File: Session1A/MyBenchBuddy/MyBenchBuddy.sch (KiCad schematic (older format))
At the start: 0 parts

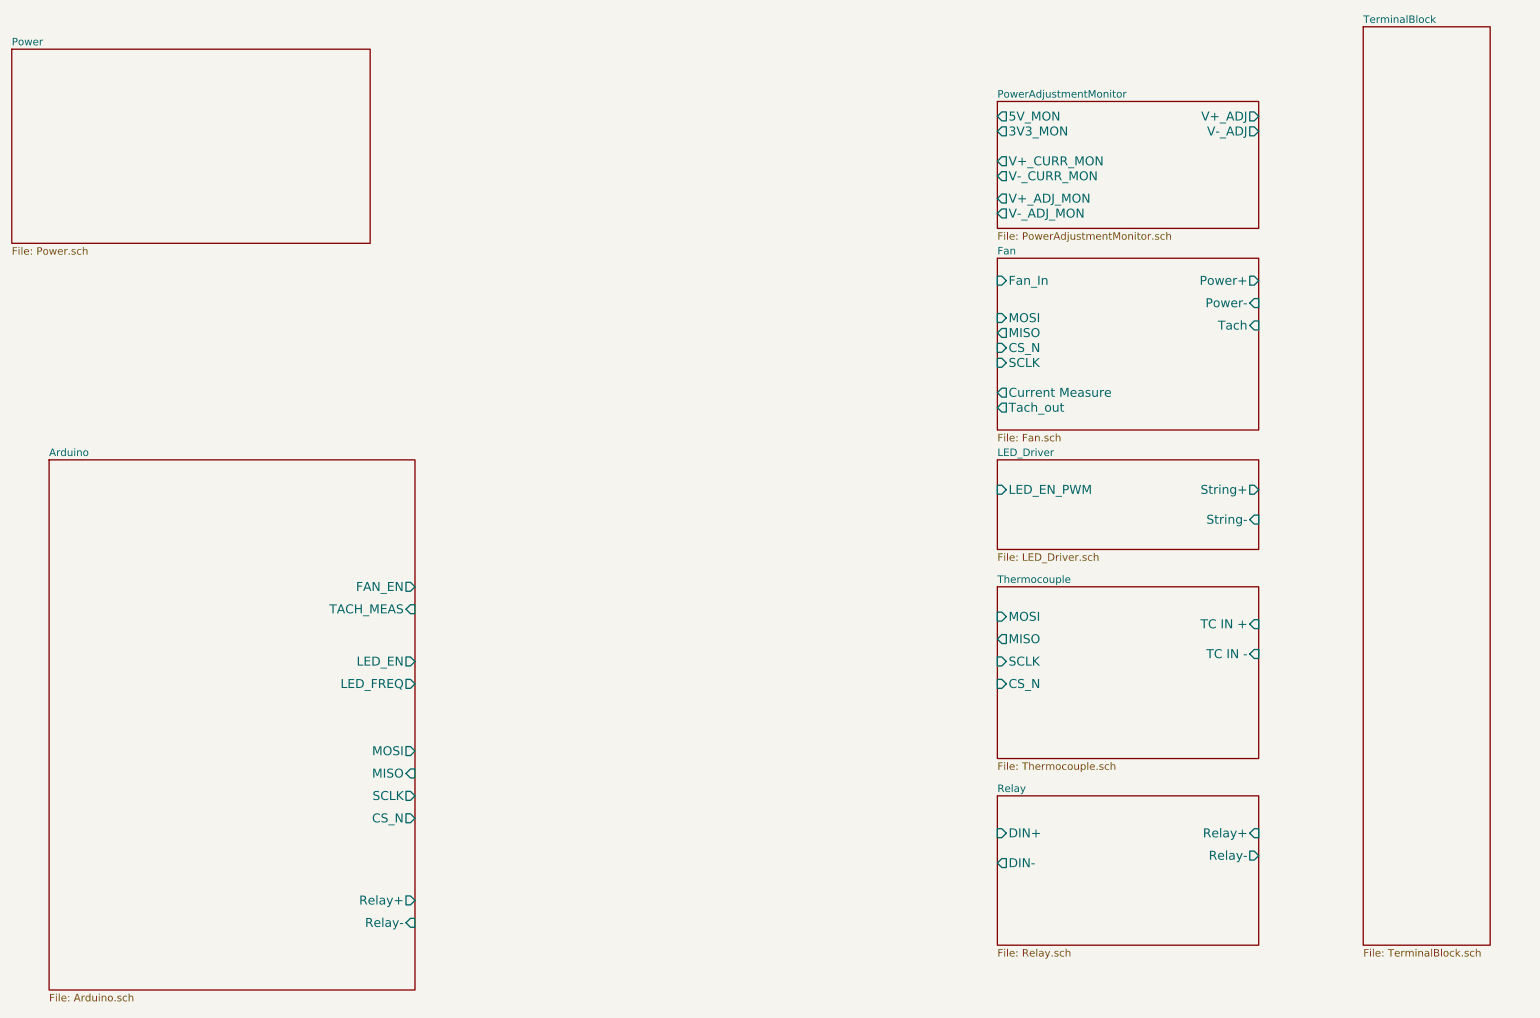
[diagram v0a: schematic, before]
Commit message: Understanding the Arduino Module
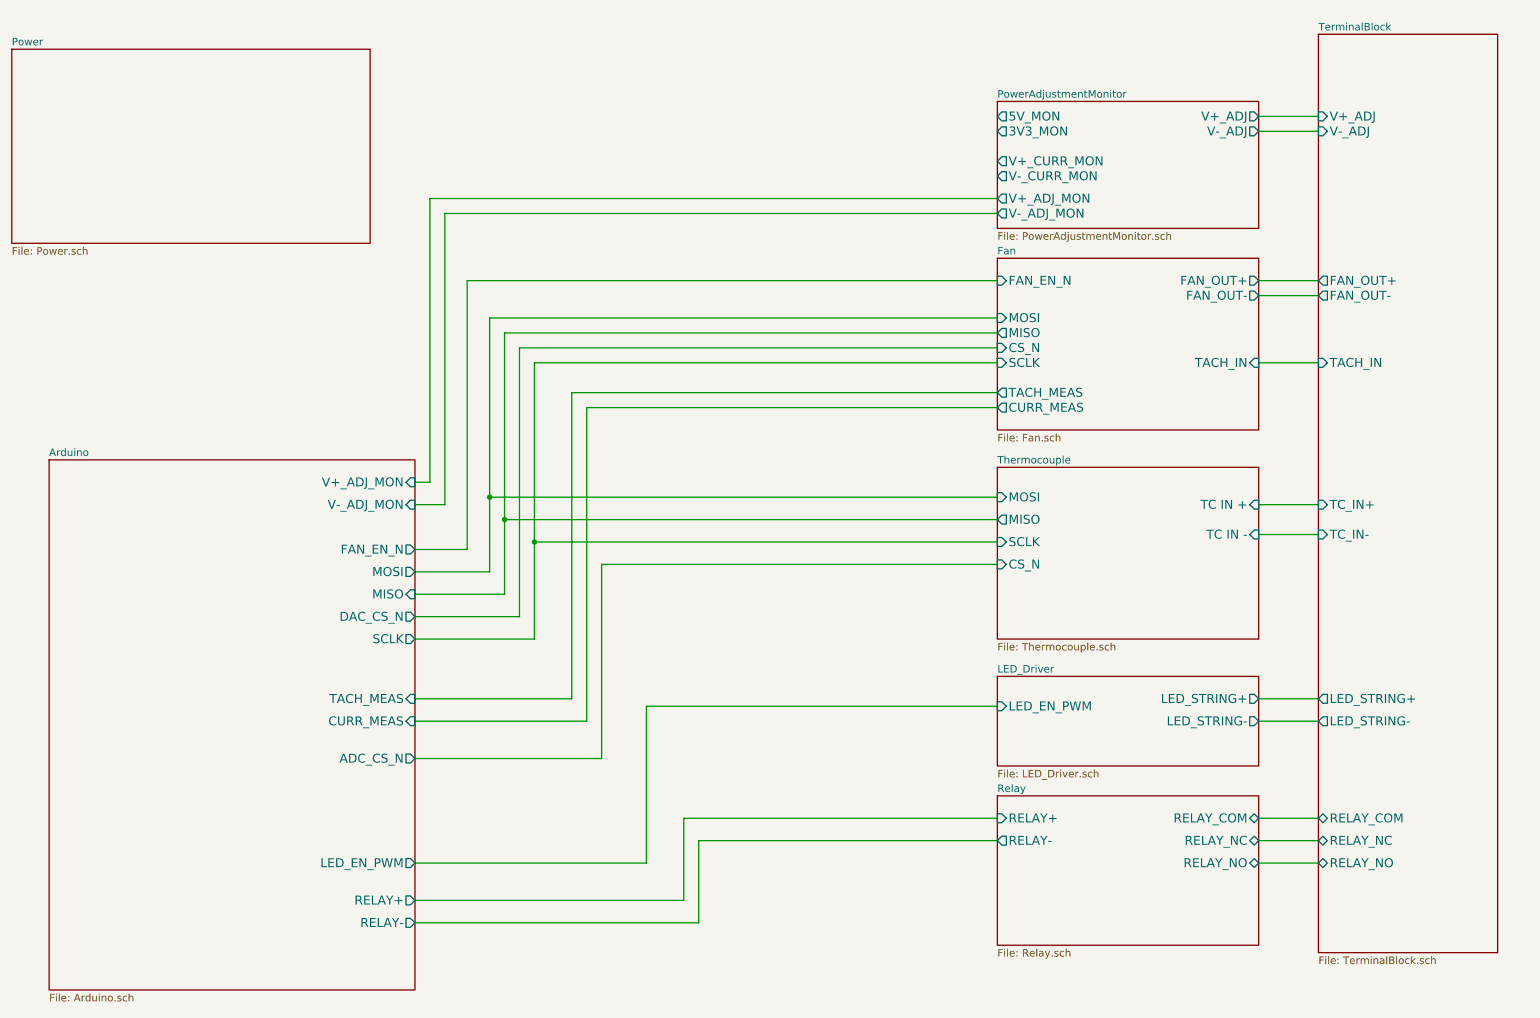
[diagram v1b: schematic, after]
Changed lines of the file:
@@
 LIBS:bth-transistor
 LIBS:bth-converter
+LIBS:bth-ic
 LIBS:MyBenchBuddy-cache
 EELAYER 27 0
@@
 Sheet 1 9
 Title ""
-Date "13 feb 2014"
+Date "26 feb 2014"
 Rev ""
 Comp ""
@@
 $EndDescr
 $Sheet
-S 1200 3650 2450 3550
-U 52EF36BC
-F0 "Arduino" 50
-F1 "Arduino.sch" 50
-F2 "Relay+" O R 3650 6600 60
-F3 "Relay-" I R 3650 6750 60
-F4 "MOSI" O R 3650 5600 60
-F5 "MISO" I R 3650 5750 60
-F6 "SCLK" O R 3650 5900 60
-F7 "CS_N" O R 3650 6050 60
-F8 "LED_EN" O R 3650 5000 60
-F9 "LED_FREQ" O R 3650 5150 60
-F10 "FAN_EN" O R 3650 4500 60
-F11 "TACH_MEAS" I R 3650 4650 60
-$EndSheet
-$Sheet
-S 7550 4500 1750 1150
-U 52EF370C
-F0 "Thermocouple" 50
-F1 "Thermocouple.sch" 50
-F2 "TC IN +" I R 9300 4750 60
-F3 "TC IN -" I R 9300 4950 60
-F4 "MOSI" I L 7550 4700 60
-F5 "MISO" O L 7550 4850 60
-F6 "SCLK" I L 7550 5000 60
-F7 "CS_N" I L 7550 5150 60
-$EndSheet
-$Sheet
 S 7550 5900 1750 1000
 U 52EF3727
 F0 "Relay" 50
 F1 "Relay.sch" 50
-F2 "DIN+" I L 7550 6150 60
-F3 "DIN-" O L 7550 6350 60
-F4 "Relay+" I R 9300 6150 60
-F5 "Relay-" O R 9300 6300 60
+F2 "RELAY_NC" B R 9300 6200 60
+F3 "RELAY_NO" B R 9300 6350 60
+F4 "RELAY_COM" B R 9300 6050 60
+F5 "RELAY+" I L 7550 6050 60
+F6 "RELAY-" O L 7550 6200 60
 $EndSheet
 $Sheet
@@
 $EndSheet
 $Sheet
-S 7550 3650 1750 600
+S 7550 5100 1750 600
 U 52EF3794
 F0 "LED_Driver" 50
 F1 "LED_Driver.sch" 50
-F2 "String+" O R 9300 3850 60
-F3 "String-" I R 9300 4050 60
-F4 "LED_EN_PWM" I L 7550 3850 60
-$EndSheet
-$Sheet
-S 7550 2300 1750 1150
-U 52EF37B6
-F0 "Fan" 50
-F1 "Fan.sch" 50
-F2 "Power+" O R 9300 2450 60
-F3 "Power-" I R 9300 2600 60
-F4 "Tach" I R 9300 2750 60
-F5 "Tach_out" O L 7550 3300 60
-F6 "Fan_In" I L 7550 2450 60
-F7 "Current Measure" O L 7550 3200 60
-F8 "MOSI" I L 7550 2700 60
-F9 "MISO" O L 7550 2800 60
-F10 "CS_N" I L 7550 2900 60
-F11 "SCLK" I L 7550 3000 60
-$EndSheet
-$Sheet
-S 10000 750  850  6150
-U 52EF37F6
-F0 "TerminalBlock" 50
-F1 "TerminalBlock.sch" 50
+F2 "LED_EN_PWM" I L 7550 5300 60
+F3 "LED_STRING+" O R 9300 5250 60
+F4 "LED_STRING-" O R 9300 5400 60
 $EndSheet
 $Sheet
@@
 F9 "V-_CURR_MON" O L 7550 1750 60
 $EndSheet
+$Sheet
+S 7550 2300 1750 1150
+U 52EF37B6
+F0 "Fan" 50
+F1 "Fan.sch" 50
+F2 "MOSI" I L 7550 2700 60
+F3 "MISO" O L 7550 2800 60
+F4 "CS_N" I L 7550 2900 60
+F5 "SCLK" I L 7550 3000 60
+F6 "FAN_OUT+" O R 9300 2450 60
+F7 "TACH_IN" I R 9300 3000 60
+F8 "TACH_MEAS" O L 7550 3200 60
+F9 "FAN_EN_N" I L 7550 2450 60
+F10 "CURR_MEAS" O L 7550 3300 60
+F11 "FAN_OUT-" O R 9300 2550 60
+$EndSheet
+Wire Wire Line
+	9300 1350 9700 1350
+Wire Wire Line
+	9700 1450 9300 1450
+Wire Wire Line
+	9300 2450 9700 2450
+Wire Wire Line
+	9700 2550 9300 2550
+Wire Wire Line
+	9300 3000 9700 3000
+Wire Wire Line
+	9300 6050 9700 6050
+Wire Wire Line
+	9700 6200 9300 6200
+Wire Wire Line
+	9300 6350 9700 6350
+$Sheet
+S 1200 3650 2450 3550
+U 52EF36BC
+F0 "Arduino" 50
+F1 "Arduino.sch" 50
+F2 "MOSI" O R 3650 4400 60
+F3 "MISO" I R 3650 4550 60
+F4 "SCLK" O R 3650 4850 60
+F5 "TACH_MEAS" I R 3650 5250 60
+F6 "RELAY+" O R 3650 6600 60
+F7 "RELAY-" O R 3650 6750 60
+F8 "FAN_EN_N" O R 3650 4250 60
+F9 "CURR_MEAS" I R 3650 5400 60
+F10 "V+_ADJ_MON" I R 3650 3800 60
+F11 "V-_ADJ_MON" I R 3650 3950 60
+F12 "LED_EN_PWM" O R 3650 6350 60
+F13 "DAC_CS_N" O R 3650 4700 60
+F14 "ADC_CS_N" O R 3650 5650 60
+$EndSheet
+Wire Wire Line
+	3650 3800 3750 3800
+Wire Wire Line
+	3750 3800 3750 1900
+Wire Wire Line
+	3750 1900 7550 1900
+Wire Wire Line
+	7550 2000 3850 2000
+Wire Wire Line
+	3850 2000 3850 3950
+Wire Wire Line
+	3850 3950 3650 3950
+Wire Wire Line
+	3650 4250 4000 4250
+Wire Wire Line
+	4000 4250 4000 2450
+Wire Wire Line
+	4000 2450 7550 2450
+Wire Wire Line
+	3650 4400 4150 4400
+Wire Wire Line
+	4150 4400 4150 2700
+Wire Wire Line
+	4150 2700 7550 2700
+Wire Wire Line
+	3650 4550 4250 4550
+Wire Wire Line
+	4250 4550 4250 2800
+Wire Wire Line
+	4250 2800 7550 2800
+Wire Wire Line
+	4350 4700 4350 2900
+Wire Wire Line
+	4350 2900 7550 2900
+Wire Wire Line
+	3650 4850 4450 4850
+Wire Wire Line
+	4450 4850 4450 3000
+Wire Wire Line
+	4450 3000 7550 3000
+Wire Wire Line
+	3650 5250 4700 5250
+Wire Wire Line
+	4700 5250 4700 3200
+Wire Wire Line
+	4700 3200 7550 3200
+Wire Wire Line
+	3650 5400 4800 5400
+Wire Wire Line
+	4800 5400 4800 3300
+Wire Wire Line
+	4800 3300 7550 3300
+$Sheet
+S 9700 800  1200 6150
+U 52EF37F6
+F0 "TerminalBlock" 50
+F1 "TerminalBlock.sch" 50
+F2 "V+_ADJ" I L 9700 1350 60
+F3 "V-_ADJ" I L 9700 1450 60
+F4 "FAN_OUT+" O L 9700 2450 60
+F5 "FAN_OUT-" O L 9700 2550 60
+F6 "TACH_IN" I L 9700 3000 60
+F7 "LED_STRING+" O L 9700 5250 60
+F8 "LED_STRING-" O L 9700 5400 60
+F9 "TC_IN+" I L 9700 3950 60
+F10 "TC_IN-" I L 9700 4150 60
+F11 "RELAY_COM" B L 9700 6050 60
+F12 "RELAY_NC" B L 9700 6200 60
+F13 "RELAY_NO" B L 9700 6350 60
+$EndSheet
+Wire Wire Line
+	9700 3950 9300 3950
+Wire Wire Line
+	9300 4150 9700 4150
+Wire Wire Line
+	9700 5250 9300 5250
+Wire Wire Line
+	9300 5400 9700 5400
+Wire Wire Line
+	7550 3900 4150 3900
+Connection ~ 4150 3900
+Wire Wire Line
+	7550 4050 4250 4050
+Connection ~ 4250 4050
+$Sheet
+S 7550 3700 1750 1150
+U 52EF370C
+F0 "Thermocouple" 50
+F1 "Thermocouple.sch" 50
+F2 "TC IN +" I R 9300 3950 60
+F3 "TC IN -" I R 9300 4150 60
+F4 "MOSI" I L 7550 3900 60
+F5 "MISO" O L 7550 4050 60
+F6 "SCLK" I L 7550 4200 60
+F7 "CS_N" I L 7550 4350 60
+$EndSheet
+Wire Wire Line
+	7550 4200 4450 4200
+Connection ~ 4450 4200
+Wire Wire Line
+	3650 5650 4900 5650
+Wire Wire Line
+	4900 5650 4900 4350
+Wire Wire Line
+	4900 4350 7550 4350
+Wire Wire Line
+	4350 4700 3650 4700
+Wire Wire Line
+	3650 6350 5200 6350
+Wire Wire Line
+	5200 6350 5200 5300
+Wire Wire Line
+	5200 5300 7550 5300
+Wire Wire Line
+	3650 6600 5450 6600
+Wire Wire Line
+	5450 6600 5450 6050
+Wire Wire Line
+	5450 6050 7550 6050
+Wire Wire Line
+	3650 6750 5550 6750
+Wire Wire Line
+	5550 6750 5550 6200
+Wire Wire Line
+	5550 6200 7550 6200
 $EndSCHEMATC
